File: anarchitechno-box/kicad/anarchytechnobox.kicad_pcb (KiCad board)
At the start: 4 copper layers, 97.2 x 116.3 mm, 102 parts, among them J2 Conn_01x03_Socket, J4 C2988369, Q1001 IRFS4310Z, Q1101 IRFS4310Z, Q1301 IRFS4310Z, Q1401 IRFS4310Z, Q201 12mhz, Q401 IRFS4310Z, Q501 IRFS4310Z, Q701 IRFS4310Z, Q801 IRFS4310Z, SW1 C318884, U1 TC4426xOA, U101 <value>, U2 ADuM1200AR, U201 TLV74311PDBVR, U21 C85364, U301 ADuM1200AR, U302 TC4426xOA, U4 LM7812_TO220, U401 ADuM1200AR, U402 TC4426xOA, U403 ADuM1200AR, U404 TC4426xOA, U6 TME-0503S, U67 LP5907MFX-3.3

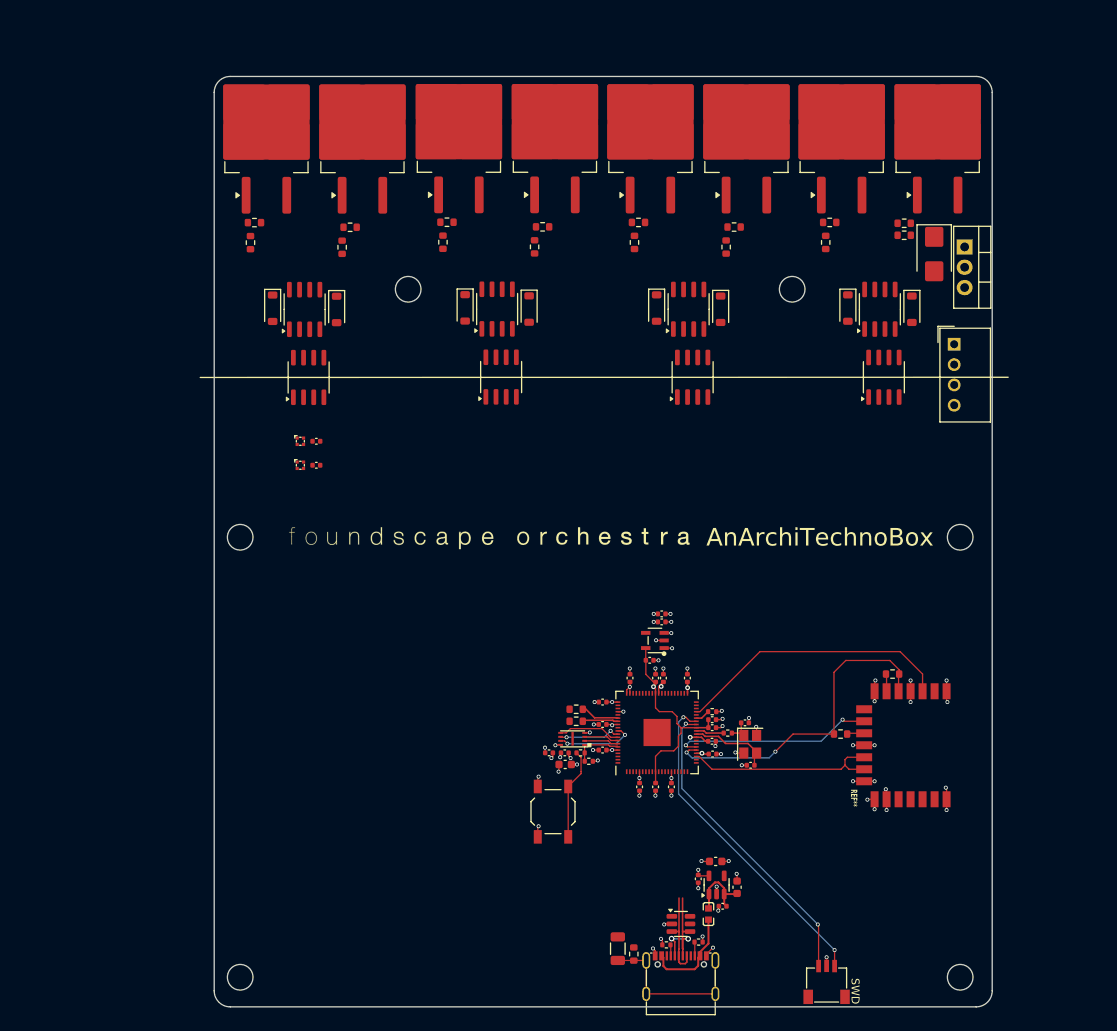
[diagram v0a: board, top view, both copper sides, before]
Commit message: Stijn in de Trein
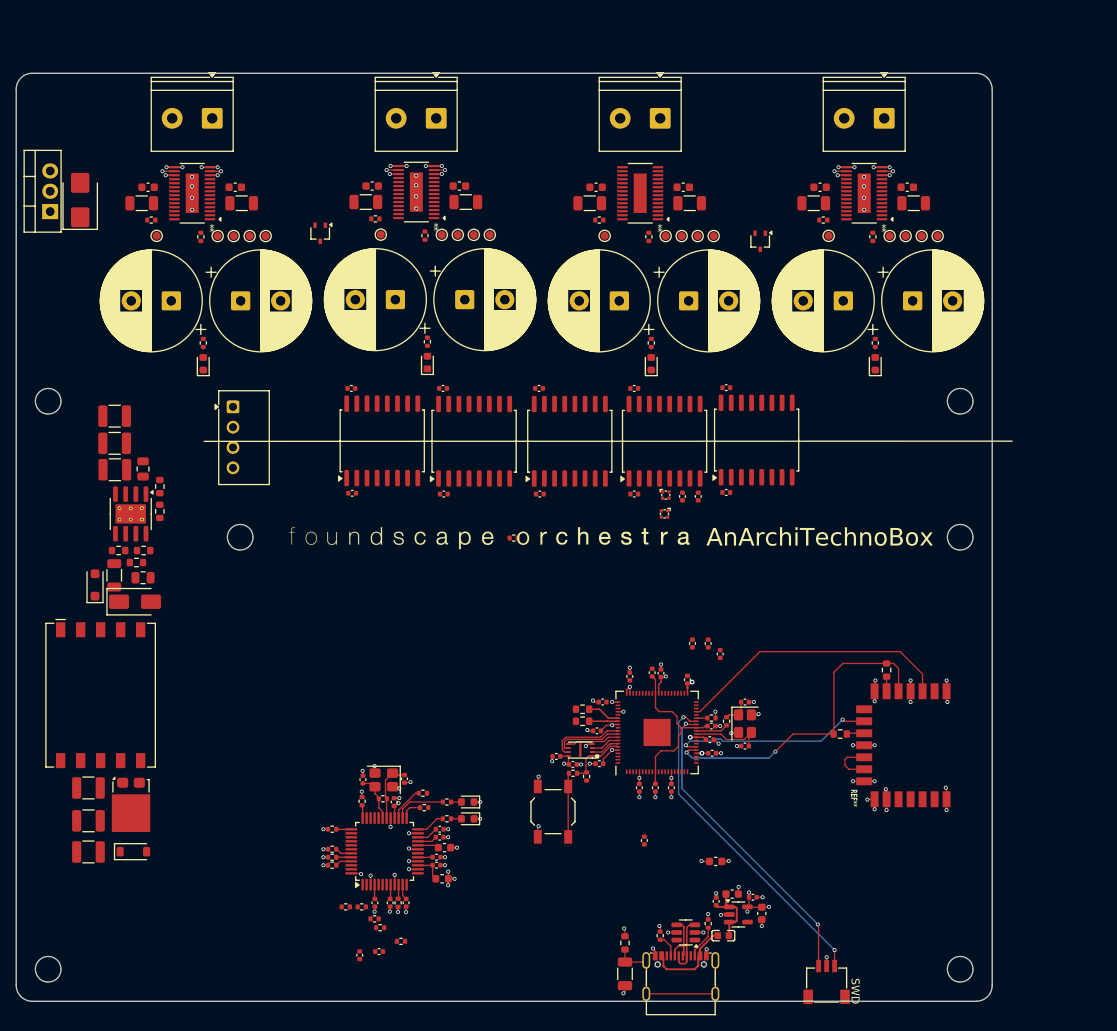
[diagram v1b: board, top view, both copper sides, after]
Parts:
- removed C101, C102: 100nF, Capacitor_SMD:C_0402_1005Metric
- removed C139, C140: 100n, Capacitor_SMD:C_0402_1005Metric
- removed C150: 4.7n 100v, Capacitor_SMD:C_1206_3216Metric
- removed D1004, D1104, D1304, D1404, D404, D504, D704, D804: MBR0530, Diode_SMD:D_SOD-123
- removed D101: C5349953, TinyLEDs:XL-1010
- removed H11, H12, H7, H8, H9: MountingHole, MountingHole:MountingHole_3.2mm_M3
- removed L3: BLM18PG121SN1D_C14709, BigFishImports:L0603
- removed Q1001, Q1101, Q1301, Q1401, Q401, Q501, Q701, Q801: IRFS4310Z, Package_TO_SOT_SMD:TO-263-2
- removed Q201: 12mhz, Crystal:Crystal_SMD_SeikoEpson_TSX3225-4Pin_3.2x2.5mm
- removed R1003, R1103, R1303, R1403, R403, R503, R703, R803: 100R, Resistor_SMD:R_0603_1608Metric
- removed R1004, R1104, R1304, R1404, R205, R404, R504, R704, R804: 10k, Resistor_SMD:R_0603_1608Metric
- removed R202: 27, Resistor_SMD:R_0603_1608Metric
- removed R204: 470, Resistor_SMD:R_0603_1608Metric
- removed U$2: C2843335 W25Q16JVUXIQ, ZephKicad:USON-8-EP(2x3)
- removed U2, U301, U401, U403: ADuM1200AR, Package_SO:SOIC-8_3.9x4.9mm_P1.27mm
- removed U201: TLV74311PDBVR, jlcpcb3:SOT-23-5_L3.0-W1.7-P0.95-LS2.8-BL
- removed U302, U402, U404: TC4426xOA, Package_SO:SOIC-8_3.9x4.9mm_P1.27mm
- removed the U4 at (137.6, 53.7)
- removed U6: TME-0503S, Converter_DCDC:Converter_DCDC_TRACO_TME_03xxS_05xxS_12xxS_Single_THT
- removed U67: LP5907MFX-3.3, Package_TO_SOT_SMD:SOT-23-5
- added C1: 100nF, Capacitor_SMD:C_0402_1005Metric, F.Cu at (102.3, 84.9)
- added C10: 1u, Capacitor_SMD:C_0402_1005Metric, F.Cu at (105.5, 103.3)
- added C11: 100nF, Capacitor_SMD:C_0402_1005Metric, F.Cu at (106.0, 117.0)
- added C12: 10uF, Capacitor_SMD:C_0603_1608Metric, F.Cu at (108.5, 134.6)
- added C13: 100nF, Capacitor_SMD:C_0402_1005Metric, F.Cu at (99.6, 107.0)
- added C15: 100nF, Capacitor_SMD:C_0402_1005Metric, F.Cu at (91.9, 118.3)
- added C17: 100n, Capacitor_SMD:C_0402_1005Metric, F.Cu at (111.1, 135.0)
- added C18: 1u, Capacitor_SMD:C_0402_1005Metric, F.Cu at (107.0, 104.6)
- added C19: 1u, Capacitor_SMD:C_0402_1005Metric, F.Cu at (97.5, 127.9)
- added C20: 10uF, Capacitor_SMD:C_0603_1608Metric, F.Cu at (112.2, 137.0)
- added C21: 100nF, Capacitor_SMD:C_0402_1005Metric, F.Cu at (105.9, 113.6)
- added C22: 100nF, Capacitor_SMD:C_0402_1005Metric, F.Cu at (98.9, 121.3)
- added C23: 100nF, Capacitor_SMD:C_0402_1005Metric, F.Cu at (98.5, 106.9)
- added C24: 4.7n 100v, Capacitor_SMD:C_1206_3216Metric, F.Cu at (95.1, 144.6)
- added C25: 0.1uF, Capacitor_SMD:C_0402_1005Metric, F.Cu at (86.5, 117.4)
- added C27: 100nF, Capacitor_SMD:C_0402_1005Metric, F.Cu at (88.6, 118.4)
- added C29: 27p, Capacitor_SMD:C_0402_1005Metric, F.Cu at (110.1, 116.1)
- added C30: 100nF, Capacitor_SMD:C_0402_1005Metric, F.Cu at (61.0, 84.5)
- added C31: 100nF, Capacitor_SMD:C_0402_1005Metric, F.Cu at (60.9, 71.4)
- added C32: 100nF, Capacitor_SMD:C_0402_1005Metric, F.Cu at (107.8, 84.4)
- added C34: 1uF 50V, Capacitor_SMD:C_0603_1608Metric, F.Cu at (130.4, 46.2)
- added C35: 1uF 50V, Capacitor_SMD:C_0603_1608Metric, F.Cu at (119.5, 46.2)
- added C36: 10uF 50V, Capacitor_SMD:C_1206_3216Metric, F.Cu at (131.2, 48.2)
- added C37: 10uF 50V, Capacitor_SMD:C_1206_3216Metric, F.Cu at (118.7, 48.2)
- added C38: 1000uF 50V, Capacitor_THT:CP_Radial_D12.5mm_P5.00mm, F.Cu at (122.4, 60.4)
- added C39: 1000uF 50V, Capacitor_THT:CP_Radial_D12.5mm_P5.00mm, F.Cu at (131.1, 60.4)
- added C40: 1uF 50V, Capacitor_SMD:C_0603_1608Metric, F.Cu at (102.4, 46.2)
- added C41: 1uF 50V, Capacitor_SMD:C_0603_1608Metric, F.Cu at (91.5, 46.2)
- added C42: 10uF 50V, Capacitor_SMD:C_1206_3216Metric, F.Cu at (103.2, 48.2)
- added C43: 10uF 50V, Capacitor_SMD:C_1206_3216Metric, F.Cu at (90.7, 48.2)
- added C44: 1000uF 50V, Capacitor_THT:CP_Radial_D12.5mm_P5.00mm, F.Cu at (94.4, 60.4)
- added C45: 1000uF 50V, Capacitor_THT:CP_Radial_D12.5mm_P5.00mm, F.Cu at (103.1, 60.4)
- added C46: 100nF, Capacitor_SMD:C_0402_1005Metric, F.Cu at (72.5, 84.6)
- added C47: 100nF, Capacitor_SMD:C_0402_1005Metric, F.Cu at (84.5, 84.6)
- added C48: 100nF, Capacitor_SMD:C_0402_1005Metric, F.Cu at (96.3, 84.6)
- added C49: 100nF, Capacitor_SMD:C_0402_1005Metric, F.Cu at (96.3, 71.4)
- added C50: 100nF, Capacitor_SMD:C_0402_1005Metric, F.Cu at (84.4, 71.4)
- added C6: 4.7u, Capacitor_SMD:C_0402_1005Metric, F.Cu at (103.5, 103.3)
- added C64: 10n, Capacitor_SMD:C_0402_1005Metric, F.Cu at (61.9, 142.2)
- added C67: 10uF 50V, Capacitor_SMD:C_1210_3225Metric, F.Cu at (31.3, 78.3)
- added C68: 1uF 25V, Capacitor_SMD:C_0805_2012Metric, F.Cu at (34.9, 81.5)
- added C69: 220pF, Capacitor_SMD:C_0805_2012Metric, F.Cu at (34.9, 95.1)
- added C7: 100nF, Capacitor_SMD:C_0402_1005Metric, F.Cu at (96.9, 121.3)
- added C70: 47uF 10V, Capacitor_SMD:C_1210_3225Metric, F.Cu at (28.0, 121.3)
- added C71: 47uF 10V, Capacitor_SMD:C_1210_3225Metric, F.Cu at (28.0, 125.5)
- added C72: 47uF 10V, Capacitor_SMD:C_1210_3225Metric, F.Cu at (28.0, 129.3)
- added C74: 1uF 50V, Capacitor_SMD:C_0603_1608Metric, F.Cu at (74.4, 46.1)
- added C75: 1uF 50V, Capacitor_SMD:C_0603_1608Metric, F.Cu at (63.5, 46.1)
- added C76: 10uF 50V, Capacitor_SMD:C_1206_3216Metric, F.Cu at (75.2, 48.1)
- added C77: 10uF 50V, Capacitor_SMD:C_1206_3216Metric, F.Cu at (62.7, 48.1)
- added C78: 1000uF 50V, Capacitor_THT:CP_Radial_D12.5mm_P5.00mm, F.Cu at (66.4, 60.3)
- added C79: 1000uF 50V, Capacitor_THT:CP_Radial_D12.5mm_P5.00mm, F.Cu at (75.1, 60.3)
- added C8: 100nF, Capacitor_SMD:C_0402_1005Metric, F.Cu at (100.9, 121.3)
- added C80: 1uF 50V, Capacitor_SMD:C_0603_1608Metric, F.Cu at (46.4, 46.2)
- added C81: 1uF 50V, Capacitor_SMD:C_0603_1608Metric, F.Cu at (35.5, 46.2)
- added C82: 10uF 50V, Capacitor_SMD:C_1206_3216Metric, F.Cu at (47.2, 48.2)
- added C83: 10uF 50V, Capacitor_SMD:C_1206_3216Metric, F.Cu at (34.7, 48.2)
- added C84: 1000uF 50V, Capacitor_THT:CP_Radial_D12.5mm_P5.00mm, F.Cu at (38.4, 60.4)
- added C85: 1000uF 50V, Capacitor_THT:CP_Radial_D12.5mm_P5.00mm, F.Cu at (47.1, 60.4)
- added C9: 100n, Capacitor_SMD:C_0402_1005Metric, F.Cu at (106.5, 135.5)
- added D10: SMAJ18A, Diode_SMD:D_SMA, F.Cu at (33.9, 98.1)
- added D11: CMMSH1-100, Diode_SMD:D_SOD-123F, F.Cu at (28.9, 96.0)
- added D12: V8PM10SHM3/I, Package_TO_SOT_SMD:TO-277A, F.Cu at (33.4, 123.5)
- added D13: CMHZ5232B, Diode_SMD:D_SOD-123, F.Cu at (33.6, 129.3)
- added D14: RED, LED_SMD:LED_0603_1608Metric, F.Cu at (70.4, 68.2)
- added D15: RED, LED_SMD:LED_0603_1608Metric, F.Cu at (42.4, 68.3)
- added D2: C5349953, TinyLEDs:XL-1010, F.Cu at (100.2, 84.7)
- added D4: BAT54AW, Package_TO_SOT_SMD:SOT-323_SC-70, F.Cu at (57.0, 52.0)
- added D5: BAT54AW, Package_TO_SOT_SMD:SOT-323_SC-70, F.Cu at (112.0, 53.0)
- added D6: RED, LED_SMD:LED_0603_1608Metric, F.Cu at (126.4, 68.3)
- added D7: RED, LED_SMD:LED_0603_1608Metric, F.Cu at (98.4, 68.3)
- added D8: RED, LED_SMD:LED_0603_1608Metric, F.Cu at (75.4, 125.2)
- added D9: RED, LED_SMD:LED_0603_1608Metric, F.Cu at (75.4, 123.1)
- added FB1: BLM18PG121SN1D, Inductor_SMD:L_0603_1608Metric, F.Cu at (72.2, 132.7)
- added H1: MountingHole, MountingHole:MountingHole_3.2mm_M3, F.Cu at (23.0, 73.0)
- added H2: MountingHole, MountingHole:MountingHole_3.2mm_M3, F.Cu at (137.0, 90.0)
- added H3: MountingHole, MountingHole:MountingHole_3.2mm_M3, F.Cu at (137.0, 73.0)
- added H4: MountingHole, MountingHole:MountingHole_3.2mm_M3, F.Cu at (137.0, 144.0)
- added H6: MountingHole, MountingHole:MountingHole_3.2mm_M3, F.Cu at (23.0, 144.0)
- added J3: Screw_Terminal_01x02, TerminalBlock_Phoenix:TerminalBlock_Phoenix_PT-1,5-2-5.0-H_1x02_P5.00mm_Horizontal, F.Cu at (71.5, 37.6)
- added J4: Screw_Terminal_01x02, TerminalBlock_Phoenix:TerminalBlock_Phoenix_PT-1,5-2-5.0-H_1x02_P5.00mm_Horizontal, F.Cu at (43.5, 37.6)
- added J5: Screw_Terminal_01x02, TerminalBlock_Phoenix:TerminalBlock_Phoenix_PT-1,5-2-5.0-H_1x02_P5.00mm_Horizontal, F.Cu at (127.5, 37.6)
- added J6: Screw_Terminal_01x02, TerminalBlock_Phoenix:TerminalBlock_Phoenix_PT-1,5-2-5.0-H_1x02_P5.00mm_Horizontal, F.Cu at (99.5, 37.6)
- added L1: BLM18PG121SN1D_C14709, BigFishImports:L0603, F.Cu at (107.4, 139.8)
- added Q1: 12mhz, Crystal:Crystal_SMD_SeikoEpson_TSX3225-4Pin_3.2x2.5mm, F.Cu at (110.1, 113.3)
- added R1: 470, Resistor_SMD:R_0603_1608Metric, F.Cu at (127.8, 106.6)
- added R10: 10k, Resistor_SMD:R_0402_1005Metric, F.Cu at (105.9, 112.6)
- added R11: 1k, Resistor_SMD:R_0402_1005Metric, F.Cu at (107.8, 113.0)
- added R12: 470R, Resistor_SMD:R_0402_1005Metric, F.Cu at (126.4, 65.7)
- added R13: 0R, Resistor_SMD:R_0402_1005Metric, F.Cu at (126.1, 52.4)
- added R14: TBD, Resistor_SMD:R_0402_1005Metric, F.Cu at (119.9, 50.3)
- added R15: 470R, Resistor_SMD:R_0402_1005Metric, F.Cu at (98.4, 65.7)
- added R16: 0R, Resistor_SMD:R_0402_1005Metric, F.Cu at (98.1, 52.4)
- added R19: 1MEG, Resistor_SMD:R_0402_1005Metric, F.Cu at (64.8, 122.7)
- added R2: 10k, Resistor_SMD:R_0603_1608Metric, F.Cu at (122.0, 114.6)
- added R20: 1K, Resistor_SMD:R_0402_1005Metric, F.Cu at (58.5, 131.0)
- added R21: 1K, Resistor_SMD:R_0402_1005Metric, F.Cu at (58.5, 130.0)
- added R22: 1K, Resistor_SMD:R_0402_1005Metric, F.Cu at (58.5, 129.0)
- added R23: 1K, Resistor_SMD:R_0402_1005Metric, F.Cu at (62.2, 123.0)
- added R24: 1K, Resistor_SMD:R_0402_1005Metric, F.Cu at (58.5, 126.5)
- added R27: 470R, Resistor_SMD:R_0402_1005Metric, F.Cu at (72.8, 123.1)
- added R29: 12.4k, Resistor_SMD:R_0402_1005Metric, F.Cu at (66.7, 135.7)
- added R3: 1M, Resistor_SMD:R_0603_1608Metric, F.Cu at (95.1, 140.7)
- added R30: 49R9, Resistor_SMD:R_0402_1005Metric, F.Cu at (62.2, 136.2)
- added R31: 49R9, Resistor_SMD:R_0402_1005Metric, F.Cu at (60.2, 136.2)
- added R32: 10R, Resistor_SMD:R_0402_1005Metric, F.Cu at (67.1, 140.5)
- added R36: 200K, Resistor_SMD:R_0603_1608Metric, F.Cu at (37.0, 83.7)
- added R37: 150K, Resistor_SMD:R_0603_1608Metric, F.Cu at (31.8, 91.7)
- added R38: 113K, Resistor_SMD:R_0603_1608Metric, F.Cu at (34.9, 91.7)
- added R39: 100R, Resistor_SMD:R_1206_3216Metric, F.Cu at (31.3, 94.8)
- added R4: 5.1k, Resistor_SMD:R_0402_1005Metric, F.Cu at (99.5, 139.8)
- added R40: 10K, Resistor_SMD:R_0603_1608Metric, F.Cu at (34.0, 93.2)
- added R41: 470R, Resistor_SMD:R_0402_1005Metric, F.Cu at (70.4, 65.6)
- added R42: 0R, Resistor_SMD:R_0402_1005Metric, F.Cu at (70.1, 52.3)
- added R43: TBD, Resistor_SMD:R_0402_1005Metric, F.Cu at (63.9, 50.2)
- added R44: 470R, Resistor_SMD:R_0402_1005Metric, F.Cu at (42.4, 65.7)
- added R45: 0R, Resistor_SMD:R_0402_1005Metric, F.Cu at (42.1, 52.4)
- added R46: TBD, Resistor_SMD:R_0402_1005Metric, F.Cu at (35.9, 50.3)
- added R5: 5.1k, Resistor_SMD:R_0402_1005Metric, F.Cu at (105.5, 138.3)
- added R6: 10k, Resistor_SMD:R_0402_1005Metric, F.Cu at (90.3, 119.9)
- added R7: 27, Resistor_SMD:R_0603_1608Metric, F.Cu at (89.8, 113.0)
- added R8: 27, Resistor_SMD:R_0603_1608Metric, F.Cu at (89.8, 111.5)
- added R9: 1k, Resistor_SMD:R_0402_1005Metric, F.Cu at (88.6, 119.5)
- added TP1: TestPoint, TestPoint:TestPoint_Pad_D1.0mm, F.Cu at (120.6, 52.3)
- added TP10: TestPoint, TestPoint:TestPoint_Pad_D1.0mm, F.Cu at (100.2, 52.3)
- added TP11: TestPoint, TestPoint:TestPoint_Pad_D1.0mm, F.Cu at (64.6, 52.2)
- added TP12: TestPoint, TestPoint:TestPoint_Pad_D1.0mm, F.Cu at (74.2, 52.2)
- added TP13: TestPoint, TestPoint:TestPoint_Pad_D1.0mm, F.Cu at (76.2, 52.2)
- added TP14: TestPoint, TestPoint:TestPoint_Pad_D1.0mm, F.Cu at (78.2, 52.2)
- added TP15: TestPoint, TestPoint:TestPoint_Pad_D1.0mm, F.Cu at (72.2, 52.2)
- added TP16: TestPoint, TestPoint:TestPoint_Pad_D1.0mm, F.Cu at (36.6, 52.3)
- added TP17: TestPoint, TestPoint:TestPoint_Pad_D1.0mm, F.Cu at (46.2, 52.3)
- added TP18: TestPoint, TestPoint:TestPoint_Pad_D1.0mm, F.Cu at (48.2, 52.3)
- added TP19: TestPoint, TestPoint:TestPoint_Pad_D1.0mm, F.Cu at (50.2, 52.3)
- added TP2: TestPoint, TestPoint:TestPoint_Pad_D1.0mm, F.Cu at (130.2, 52.3)
- added TP20: TestPoint, TestPoint:TestPoint_Pad_D1.0mm, F.Cu at (44.2, 52.3)
- added TP3: TestPoint, TestPoint:TestPoint_Pad_D1.0mm, F.Cu at (132.2, 52.3)
- added TP4: TestPoint, TestPoint:TestPoint_Pad_D1.0mm, F.Cu at (134.2, 52.3)
- added TP5: TestPoint, TestPoint:TestPoint_Pad_D1.0mm, F.Cu at (128.2, 52.3)
- added TP6: TestPoint, TestPoint:TestPoint_Pad_D1.0mm, F.Cu at (92.6, 52.3)
- added TP7: TestPoint, TestPoint:TestPoint_Pad_D1.0mm, F.Cu at (102.2, 52.3)
- added TP8: TestPoint, TestPoint:TestPoint_Pad_D1.0mm, F.Cu at (104.2, 52.3)
- added TP9: TestPoint, TestPoint:TestPoint_Pad_D1.0mm, F.Cu at (106.2, 52.3)
- added U$1: C2843335 W25Q16JVUXIQ, ZephKicad:USON-8-EP(2x3), F.Cu at (89.5, 116.6)
- added U10: ISO7740DWR, Package_SO:SOIC-16W_7.5x10.3mm_P1.27mm, F.Cu at (111.6, 77.8)
- added U11: DRV8243SQDGQRQ1, parts:TI_HVSSOP-28, F.Cu at (125.0, 47.0)
- added U12: DRV8243SQDGQRQ1, parts:TI_HVSSOP-28, F.Cu at (97.0, 47.0)
- added U13: ISO7740DWR, Package_SO:SOIC-16W_7.5x10.3mm_P1.27mm, F.Cu at (76.2, 78.0)
- added U14: ISO7740DWR, Package_SO:SOIC-16W_7.5x10.3mm_P1.27mm, F.Cu at (88.2, 78.0)
- added U15: ISO7742DWR, Package_SO:SOIC-16W_7.5x10.3mm_P1.27mm, F.Cu at (100.0, 78.0)
- added U16: W5500, Package_QFP:LQFP-48_7x7mm_P0.5mm, F.Cu at (65.0, 129.3)
- added U18: ADPL54203ES8E#PBF, Package_SO:SOIC-8-1EP_3.9x4.9mm_P1.27mm_EP2.41x3.81mm_ThermalVias, F.Cu at (33.3, 87.1)
- added U19: 750311564, parts:T_Wurth_WE-FB-EP13_16.36, F.Cu at (29.6, 109.7)
- added U20: DRV8243SQDGQRQ1, parts:TI_HVSSOP-28, F.Cu at (69.0, 46.9)
- added U3: LM7812_TO220, Package_TO_SOT_THT:TO-220-3_Vertical, F.Cu at (23.2, 49.3)
- added U5: LP5907MFX-3.3, Package_TO_SOT_SMD:SOT-23-5, F.Cu at (109.3, 137.2)
- added U7: C85364, Package_TO_SOT_SMD:SOT-23-6, F.Cu at (102.7, 139.4)
- added U9: ISO7740DWR, Package_SO:SOIC-16W_7.5x10.3mm_P1.27mm, F.Cu at (64.8, 78.0)
- added Y1: 25MHz, Crystal:Crystal_SMD_3225-4Pin_3.2x2.5mm, F.Cu at (65.0, 120.3)
- C14: value 0.1uF -> 100nF
- C16: value 10uF -> 100nF; footprint Capacitor_SMD:C_0603_1608Metric -> Capacitor_SMD:C_0402_1005Metric
- C28: value 10uF -> 27p; footprint Capacitor_SMD:C_0603_1608Metric -> Capacitor_SMD:C_0402_1005Metric
- C3, C5, C60: value 1u -> 100nF
- C52, C53: value 100nF -> 15p
- C57: value 100nF -> 10nF
- C59: value 4.7u -> 4.7uF; footprint Capacitor_SMD:C_0402_1005Metric -> Capacitor_SMD:C_0603_1608Metric
- C63: value 100nF -> 22n
- C65: value 27p -> 330uF 50V; footprint Capacitor_SMD:C_0402_1005Metric -> Capacitor_SMD:C_1210_3225Metric
- C66: value 27p -> 10uF 50V; footprint Capacitor_SMD:C_0402_1005Metric -> Capacitor_SMD:C_1210_3225Metric
- D1: value C5349953 -> SM6T24A; footprint TinyLEDs:XL-1010 -> Diode_SMD:D_SMB
- D3: value SM6T24A -> C5349953; footprint Diode_SMD:D_SMB -> TinyLEDs:XL-1010
- R17: value 10k -> TBD
- R18: value 1k -> 10K
- R25: value 10k -> 470R
- R26: value 1k -> 470R
- R28: value 27 -> 470R; footprint Resistor_SMD:R_0603_1608Metric -> Resistor_SMD:R_0402_1005Metric
- R33: value 1M -> 49R9; footprint Resistor_SMD:R_0603_1608Metric -> Resistor_SMD:R_0402_1005Metric
- R34: value 5.1k -> 49R9
- R35: value 5.1k -> 1MEG; footprint Resistor_SMD:R_0402_1005Metric -> Resistor_SMD:R_0603_1608Metric
- U1: value TC4426xOA -> TME-0503S; footprint Package_SO:SOIC-8_3.9x4.9mm_P1.27mm -> Converter_DCDC:Converter_DCDC_TRACO_TME_03xxS_05xxS_12xxS_Single_THT
- U21: value C85364 -> DRV8243SQDGQRQ1; footprint Package_TO_SOT_SMD:SOT-23-6 -> parts:TI_HVSSOP-28
- moved U21 109.9 mm to (41.0, 47.0), turned to 180 degrees
- moved C66 87.6 mm to (31.3, 81.6)
- moved C65 87.6 mm to (31.3, 74.9), turned to 180 degrees
- moved R35 86.2 mm to (37.0, 86.8), turned to -90 degrees
- moved R17 63.1 mm to (91.9, 50.3)
- moved C61 47.5 mm to (63.8, 135.7), turned to -90 degrees
- moved D3 46.8 mm to (100.0, 87.1)
- moved C60 46.3 mm to (65.7, 135.7), turned to -90 degrees
- moved C51 43.1 mm to (72.4, 71.4), turned to 0 degrees
- moved D1 43.1 mm to (27.0, 47.8), turned to 90 degrees
- moved C59 39.9 mm to (72.5, 128.8), turned to 0 degrees
- moved C55 37.4 mm to (71.5, 130.0), turned to 0 degrees
- moved C33 37.4 mm to (107.8, 71.3), turned to 0 degrees
- moved R34 36.6 mm to (63.8, 137.7), turned to 0 degrees
- moved R18 36.2 mm to (81.2, 90.1)
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- renumbered J4 to J1, U101 to U4, U3 to U8
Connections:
- C14 pad 1: +3V3 -> GND
- C14 pad 2: GND -> +3V3
- C16 pad 1: +3V3 -> GND
- C16 pad 2: GND -> +3V3
- C28 pad 1: /RP2350BMCU/5V_filtered -> Net-(Q1-X1)
- C33 pad 1: GND -> +3.3VP
- C33 pad 2: +1V1 -> GND2
- C5 pad 2: +1V1 -> +3V3
- C51 pad 1: GND -> +3.3VP
- C51 pad 2: +3V3 -> GND2
- C52 pad 1: GND -> Net-(U16-XI/CLKIN)
- C52 pad 2: +3V3 -> GND
- C53 pad 1: GND -> Net-(U16-XO)
- C53 pad 2: +3V3 -> GND
- C54 pad 1: GND -> +3V3
- C54 pad 2: +3V3 -> GND
- C55 pad 1: GND -> +3.3VA
- C55 pad 2: +3V3 -> GND
- C56 pad 1: GND -> +3.3VA
- C56 pad 2: +3V3 -> GND
- C57 pad 1: GND -> Net-(U16-1V2O)
- C57 pad 2: +3V3 -> GND
- C58 pad 1: GND -> +3.3VA
- C58 pad 2: +3V3 -> GND
- C59 pad 1: +3V3 -> Net-(U16-TOCAP)
- C60 pad 1: +1V1 -> +3.3VA
- C61 pad 1: +1V1 -> +3.3VA
- C62 pad 1: +1V1 -> +3.3VA
- C63 pad 2: +3V3 -> Net-(U17-TCT)
- C65 pad 1: Net-(Q201-X1) -> +VDC
- C65 pad 2: GND -> GND2
- C66 pad 1: Net-(Q201-X2) -> +VDC
- C66 pad 2: GND -> GND2
- D1 pad 1: Net-(D1-DO) -> +24V
- D1 pad 2: +3V3 -> GND2
- D3 pad 1: +24V -> unconnected-(D3-DO-Pad1)
- D3 pad 2: GND2 -> +3V3
- J1 pad A5: Net-(J4-CC1) -> Net-(J1-CC1)
- J1 pad B5: Net-(J4-CC2) -> Net-(J1-CC2)
- J1 pad SHELL1: Net-(C150-Pad2) -> Net-(C24-Pad2)
- J1 pad SHELL2: Net-(C150-Pad2) -> Net-(C24-Pad2)
- J1 pad SHELL3: Net-(C150-Pad2) -> Net-(C24-Pad2)
- J1 pad SHELL4: Net-(C150-Pad2) -> Net-(C24-Pad2)
- R17 pad 1: +3V3 -> /TwoIsolatedFETs1/HBridge_B/DRV_ISENSE
- R17 pad 2: /RP2350BMCU/RUN -> GND2
- R18 pad 1: Net-(Q201-X1) -> +3.3VP
- R18 pad 2: Net-(U3-XOUT) -> /Isolators/PWR_DRV_nFAULT_COMMON
- R25 pad 1: /RP2350BMCU/MEM_CS -> Net-(U16-SPDLED)
- R25 pad 2: +3V3 -> Net-(D8-A)
- R26 pad 1: /RP2350BMCU/MEM_CS -> Net-(U16-LINKLED)
- R26 pad 2: /RP2350BMCU/BOOTSEL_BUT -> Net-(U17-LEDG_A)
- R28 pad 1: /RP2350BMCU/USB_N -> Net-(U16-ACTLED)
- R28 pad 2: /RP2350BMCU/USB_PRE_N -> Net-(U17-LEDY_A)
- R33 pad 1: GND -> +3.3V
- R33 pad 2: Net-(C150-Pad2) -> /Ethernet/ETH_RX_P
- R34 pad 1: Net-(J4-CC1) -> +3.3V
- R34 pad 2: GND -> /Ethernet/ETH_RX_M
- R35 pad 1: Net-(J4-CC2) -> Net-(R35-+)
- R35 pad 2: GND -> +VDC
- U1 pad 1: unconnected-(U1-NC-Pad1) -> GND2
- U1 pad 2: Net-(U1-IN_A) -> +5V
- U1 pad 3: unconnected-(U1-GND-Pad3) -> GND
- U1 pad 4: Net-(U1-IN_B) -> +3.3V
- U21 pad 1: unconnected-(U21-IO1-Pad1) -> /Isolators/PWR_SPI_CLK
- U21 pad 2: GND -> /Isolators/PWR_SPI_CS2
- U21 pad 3: /RP2350BMCU/USB_P -> /TwoIsolatedFETs0/HBridge_B/PWM_2
- U21 pad 4: /RP2350BMCU/USB_N -> /TwoIsolatedFETs0/HBridge_B/PWM_1
- U21 pad 5: +3V3 -> /Isolators/PWR_PWM_B_OFF
- U21 pad 6: unconnected-(U21-IO4-Pad6) -> +VDC
- U8 pad 1: unconnected-(U3-GPIO4-Pad1) -> /RP2350BMCU/PWM2_A
- U8 pad 11: unconnected-(U3-GPIO12-Pad11) -> /RP2350BMCU/PWM6_A
- U8 pad 13: unconnected-(U3-GPIO14-Pad13) -> /RP2350BMCU/PWM7_A
- U8 pad 19: unconnected-(U3-GPIO19-Pad19) -> /Ethernet/SPI_MOSI
- U8 pad 20: unconnected-(U3-GPIO20-Pad20) -> /Ethernet/SPI_MISO
- U8 pad 21: unconnected-(U3-GPIO21-Pad21) -> /Ethernet/SPI_CS
- U8 pad 22: unconnected-(U3-GPIO22-Pad22) -> /Ethernet/SPI_SCK
- U8 pad 28: unconnected-(U3-GPIO27-Pad28) -> /Isolators/MCU_SPI_CLK
- U8 pad 3: unconnected-(U3-GPIO6-Pad3) -> /RP2350BMCU/PWM3_A
- U8 pad 30: Net-(Q201-X2) -> Net-(Q1-X2)
- U8 pad 31: Net-(U3-XOUT) -> Net-(U8-XOUT)
- U8 pad 36: unconnected-(U3-GPIO28-Pad36) -> /Isolators/MCU_SPI_MOSI
- U8 pad 38: unconnected-(U3-GPIO30-Pad38) -> /Isolators/MCU_SPI_MISO
- U8 pad 39: unconnected-(U3-GPIO31-Pad39) -> /Isolators/MCU_DRV_nFAULT_COMMON
- U8 pad 40: unconnected-(U3-GPIO32-Pad40) -> /RP2350BMCU/I2C0_SCL
- U8 pad 42: unconnected-(U3-GPIO33-Pad42) -> /RP2350BMCU/I2C0_SDA
- U8 pad 43: unconnected-(U3-GPIO34-Pad43) -> /RP2350BMCU/UART0_TX
- U8 pad 44: unconnected-(U3-GPIO35-Pad44) -> /RP2350BMCU/UART0_RX
- U8 pad 45: unconnected-(U3-GPIO36-Pad45) -> /RP2350BMCU/UART1_TX
- U8 pad 46: unconnected-(U3-GPIO37-Pad46) -> /RP2350BMCU/UART1_RX
- U8 pad 47: unconnected-(U3-GPIO38-Pad47) -> /RP2350BMCU/I2C1_SCL
- U8 pad 48: unconnected-(U3-GPIO39-Pad48) -> /RP2350BMCU/I2C1_SDA
- U8 pad 49: unconnected-(U3-GPIO40_ADC0-Pad49) -> /Isolators/MCU_PWM_A_OFF
- U8 pad 52: unconnected-(U3-GPIO41_ADC1-Pad52) -> /Isolators/MCU_CS1
- U8 pad 53: unconnected-(U3-GPIO42_ADC2-Pad53) -> /Isolators/MCU_PWM_B_OFF
- U8 pad 54: unconnected-(U3-GPIO43_ADC3-Pad54) -> /Isolators/MCU_CS2
- U8 pad 55: unconnected-(U3-GPIO44_ADC4-Pad55) -> /Isolators/MCU_PWM_C_OFF
- U8 pad 56: unconnected-(U3-GPIO45_ADC5-Pad56) -> /Isolators/MCU_CS3
- U8 pad 57: unconnected-(U3-GPIO46_ADC6-Pad57) -> /Isolators/MCU_PWM_D_OFF
- U8 pad 58: unconnected-(U3-GPIO47_ADC7-Pad58) -> /Isolators/MCU_CS4
- U8 pad 6: unconnected-(U3-GPIO8-Pad6) -> /RP2350BMCU/PWM4_A
- U8 pad 77: unconnected-(U3-GPIO0-Pad77) -> /RP2350BMCU/PWM0_A
- U8 pad 78: unconnected-(U3-GPIO1-Pad78) -> /LED_STRING
- U8 pad 79: /LED_STRING -> /RP2350BMCU/PMW1_A
- U8 pad 8: unconnected-(U3-GPIO10-Pad8) -> /RP2350BMCU/PWM5_A
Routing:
- net GND2: track 0.00 -> 26.8 mm, vias 0 -> 36
- net Net-(C24-Pad2): track 0.00 -> 21.0 mm
- net Net-(C150-Pad2): track 20.6 -> 0.00 mm
- net /RP2350BMCU/WIFI_23: track 25.3 -> 5.83 mm
- net GND: track 47.0 -> 63.7 mm, vias 51 -> 70
- net +3.3VA: track 0.00 -> 13.4 mm
- net Net-(Q201-X2): track 10.2 -> 0.00 mm
- net +3V3: track 33.9 -> 43.3 mm, vias 27 -> 31
- net Net-(Q1-X2): track 0.00 -> 8.92 mm
- net /RP2350BMCU/USB_N: track 14.5 -> 6.79 mm, vias 2 -> 0
- net Net-(U16-XI/CLKIN): track 0.00 -> 7.01 mm
- net Net-(U16-DUPLED): track 0.00 -> 6.51 mm
- net Net-(U16-XO): track 0.00 -> 5.25 mm
- net +1V1: track 26.7 -> 21.5 mm, vias 1 -> 0
- net Net-(U16-ACTLED): track 0.00 -> 4.39 mm
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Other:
- board size 97.2 x 116.3 mm -> 122 x 116 mm

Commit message: meer Stijn in de Trein
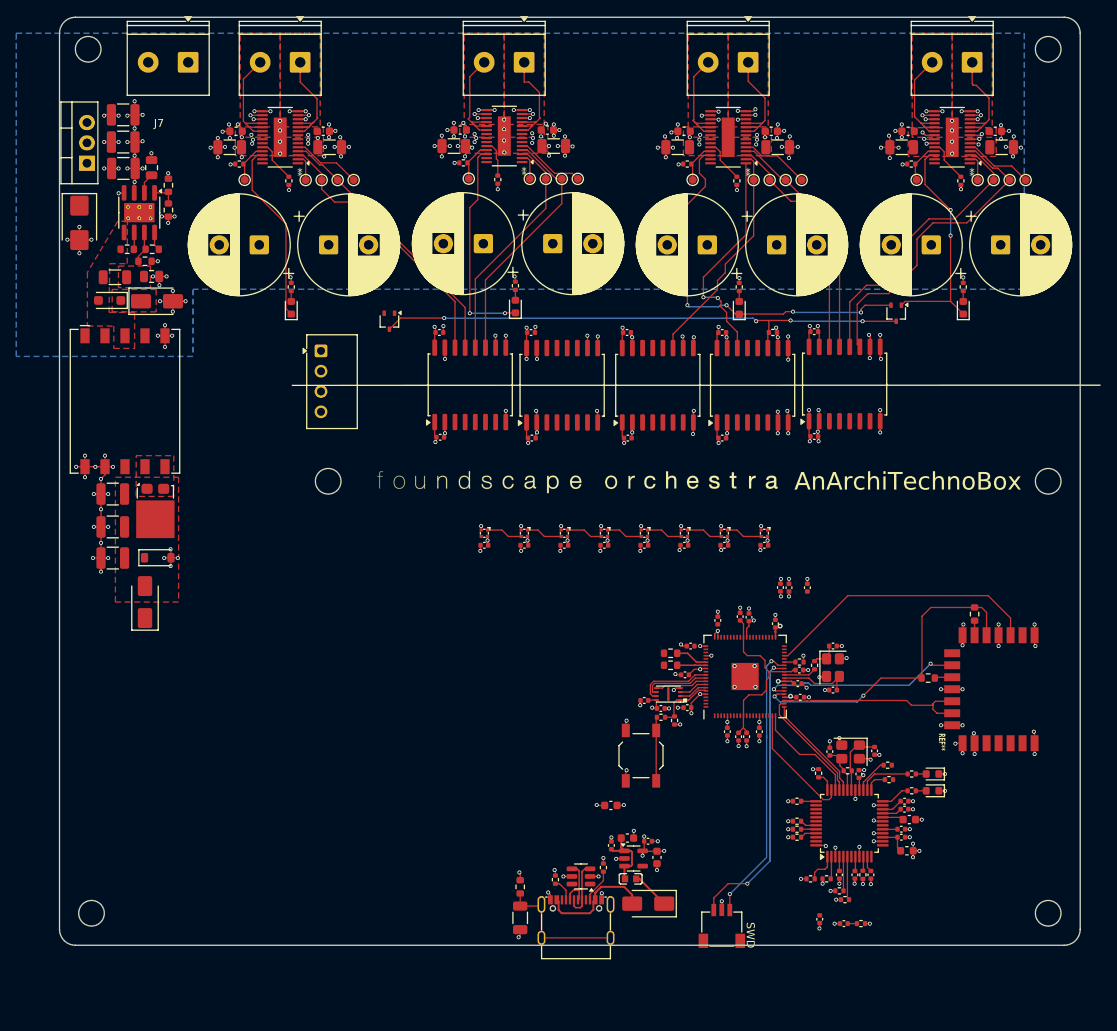
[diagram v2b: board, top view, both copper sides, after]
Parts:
- added C86: 100nF, Capacitor_SMD:C_0402_1005Metric, F.Cu at (87.5, 91.0)
- added C87: 100nF, Capacitor_SMD:C_0402_1005Metric, F.Cu at (92.5, 91.0)
- added C88: 100nF, Capacitor_SMD:C_0402_1005Metric, F.Cu at (97.5, 91.0)
- added C89: 100nF, Capacitor_SMD:C_0402_1005Metric, F.Cu at (102.5, 91.0)
- added C90: 100nF, Capacitor_SMD:C_0402_1005Metric, F.Cu at (107.5, 91.0)
- added C91: 100nF, Capacitor_SMD:C_0402_1005Metric, F.Cu at (112.5, 91.0)
- added D16: SS34, Diode_SMD:D_SMA, F.Cu at (98.0, 135.8)
- added D17: SS34, Diode_SMD:D_SMA, F.Cu at (35.1, 98.1)
- added D18: C5349953, TinyLEDs:XL-1010, F.Cu at (87.5, 89.5)
- added D19: C5349953, TinyLEDs:XL-1010, F.Cu at (92.5, 89.5)
- added D20: C5349953, TinyLEDs:XL-1010, F.Cu at (97.5, 89.5)
- added D21: C5349953, TinyLEDs:XL-1010, F.Cu at (102.5, 89.5)
- added D22: C5349953, TinyLEDs:XL-1010, F.Cu at (107.5, 89.5)
- added D23: C5349953, TinyLEDs:XL-1010, F.Cu at (112.5, 89.5)
- added J7: Screw_Terminal_01x02, TerminalBlock_Phoenix:TerminalBlock_Phoenix_PT-1,5-2-5.0-H_1x02_P5.00mm_Horizontal, F.Cu at (40.5, 30.6)
- moved C52 58.9 mm to (126.3, 116.7)
- moved C53 58.5 mm to (120.7, 116.8)
- moved Y1 58.5 mm to (123.3, 116.8)
- moved C54 58.2 mm to (124.3, 119.6)
- moved C58 58.2 mm to (125.8, 132.2)
- moved C60 58.2 mm to (123.8, 132.2)
- moved C63 58.2 mm to (122.5, 138.3)
- moved FB1 58.2 mm to (130.3, 129.2)
- moved R29 58.2 mm to (124.8, 132.2)
- moved R34 58.2 mm to (121.9, 134.2)
- moved U16 58.2 mm to (123.2, 125.8)
- moved C56 58.2 mm to (130.0, 124.0)
- moved C57 58.2 mm to (130.0, 123.0)
- moved D8 58.2 mm to (133.5, 121.7)
- moved D9 58.2 mm to (133.5, 119.6)
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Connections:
- net /TwoIsolatedFETs0/OUTPUT_A renamed /HB_1_OUT_A
- net /TwoIsolatedFETs0/OUTPUT_B renamed /HB_1_OUT_B
- net /TwoIsolatedFETs0/OUTPUT_C renamed /HB_1_OUT_C
- net /TwoIsolatedFETs0/OUTPUT_D renamed /HB_1_OUT_D
- net /TwoIsolatedFETs1/OUTPUT_A renamed /HB_2_OUT_A
- net /TwoIsolatedFETs1/OUTPUT_B renamed /HB_2_OUT_B
- net /TwoIsolatedFETs1/OUTPUT_C renamed /HB_2_OUT_C
- net /TwoIsolatedFETs1/OUTPUT_D renamed /HB_2_OUT_D
- net Net-(C69--) renamed /DCDC Flyback/VDC_CAPRES
- net Net-(D10-K) renamed /DCDC Flyback/VDC_DIODES
- net Net-(D11-A) renamed /DCDC Flyback/VDC_SW
- net Net-(D12-A-Pad1) renamed /DCDC Flyback/PRE_PRE_5V
- C30 pad 1: +3.3V -> +3V3
- C32 pad 1: +3.3V -> +3V3
- C46 pad 1: +3.3V -> +3V3
- C47 pad 1: +3.3V -> +3V3
- C48 pad 1: +3.3V -> +3V3
- C70 pad 1: +5V -> /DCDC Flyback/PRE_5V
- C71 pad 1: +5V -> /DCDC Flyback/PRE_5V
- C72 pad 1: +5V -> /DCDC Flyback/PRE_5V
- D12 pad 3: +5V -> /DCDC Flyback/PRE_5V
- D13 pad 1: +5V -> /DCDC Flyback/PRE_5V
- D14 pad 1: /TwoIsolatedFETs0/HBridge_A/DRV_nFAULT -> /TwoIsolatedFETs0/HBridge_B/DRV_nFAULT
- D15 pad 1: /TwoIsolatedFETs0/HBridge_B/DRV_nFAULT -> /TwoIsolatedFETs0/HBridge_A/DRV_nFAULT
- D3 pad 1: unconnected-(D3-DO-Pad1) -> Net-(D18-DI)
- D4 pad 1: /TwoIsolatedFETs0/HBridge_A/DRV_nFAULT -> /TwoIsolatedFETs0/HBridge_B/DRV_nFAULT
- D4 pad 2: /TwoIsolatedFETs0/HBridge_B/DRV_nFAULT -> /TwoIsolatedFETs0/HBridge_A/DRV_nFAULT
- D5 pad 1: /TwoIsolatedFETs1/HBridge_A/DRV_nFAULT -> /TwoIsolatedFETs1/HBridge_B/DRV_nFAULT
- D5 pad 2: /TwoIsolatedFETs1/HBridge_B/DRV_nFAULT -> /TwoIsolatedFETs1/HBridge_A/DRV_nFAULT
- D6 pad 1: /TwoIsolatedFETs1/HBridge_A/DRV_nFAULT -> /TwoIsolatedFETs1/HBridge_B/DRV_nFAULT
- D7 pad 1: /TwoIsolatedFETs1/HBridge_B/DRV_nFAULT -> /TwoIsolatedFETs1/HBridge_A/DRV_nFAULT
- J1 pad A4B9: +5V -> /RP2350BMCU/BREAKOUT_5V
- J1 pad A9B4: +5V -> /RP2350BMCU/BREAKOUT_5V
- R14 pad 1: /TwoIsolatedFETs1/HBridge_A/DRV_ISENSE -> /TwoIsolatedFETs1/HBridge_B/DRV_ISENSE
- R17 pad 1: /TwoIsolatedFETs1/HBridge_B/DRV_ISENSE -> /TwoIsolatedFETs1/HBridge_A/DRV_ISENSE
- R30 pad 1: +3.3V -> +3V3
- R31 pad 1: +3.3V -> +3V3
- R32 pad 1: +3.3V -> +3V3
- R33 pad 1: +3.3V -> +3V3
- R34 pad 1: +3.3V -> +3V3
- R43 pad 1: /TwoIsolatedFETs0/HBridge_A/DRV_ISENSE -> /TwoIsolatedFETs0/HBridge_B/DRV_ISENSE
- R46 pad 1: /TwoIsolatedFETs0/HBridge_B/DRV_ISENSE -> /TwoIsolatedFETs0/HBridge_A/DRV_ISENSE
- TP1 pad 1: /TwoIsolatedFETs1/HBridge_A/DRV_ISENSE -> /TwoIsolatedFETs1/HBridge_B/DRV_ISENSE
- TP11 pad 1: /TwoIsolatedFETs0/HBridge_A/DRV_ISENSE -> /TwoIsolatedFETs0/HBridge_B/DRV_ISENSE
- TP12 pad 1: /TwoIsolatedFETs0/HBridge_A/PWM_2 -> /TwoIsolatedFETs0/PWM_B_2
- TP13 pad 1: /TwoIsolatedFETs0/HBridge_A/PWM_1 -> /TwoIsolatedFETs0/PWM_B_1
- TP14 pad 1: /Isolators/PWR_PWM_A_OFF -> /Isolators/PWR_PWM_B_OFF
- TP16 pad 1: /TwoIsolatedFETs0/HBridge_B/DRV_ISENSE -> /TwoIsolatedFETs0/HBridge_A/DRV_ISENSE
- TP17 pad 1: /TwoIsolatedFETs0/HBridge_B/PWM_2 -> /TwoIsolatedFETs0/PWM_A_2
- TP18 pad 1: /TwoIsolatedFETs0/HBridge_B/PWM_1 -> /TwoIsolatedFETs0/PWM_A_1
- TP19 pad 1: /Isolators/PWR_PWM_B_OFF -> /Isolators/PWR_PWM_A_OFF
- TP2 pad 1: /TwoIsolatedFETs1/HBridge_A/PWM_2 -> /TwoIsolatedFETs1/PWM_B_2
- TP3 pad 1: /TwoIsolatedFETs1/HBridge_A/PWM_1 -> /TwoIsolatedFETs1/PWM_B_1
- TP4 pad 1: /Isolators/PWR_PWM_C_OFF -> /Isolators/PWR_PWM_D_OFF
- TP6 pad 1: /TwoIsolatedFETs1/HBridge_B/DRV_ISENSE -> /TwoIsolatedFETs1/HBridge_A/DRV_ISENSE
- TP7 pad 1: /TwoIsolatedFETs1/HBridge_B/PWM_2 -> /TwoIsolatedFETs1/PWM_A_2
- TP8 pad 1: /TwoIsolatedFETs1/HBridge_B/PWM_1 -> /TwoIsolatedFETs1/PWM_A_1
- TP9 pad 1: /Isolators/PWR_PWM_D_OFF -> /Isolators/PWR_PWM_C_OFF
- U10 pad 1: +3.3V -> +3V3
- U10 pad 11: /TwoIsolatedFETs1/HBridge_B/PWM_2 -> /TwoIsolatedFETs1/PWM_B_1
- U10 pad 12: /TwoIsolatedFETs1/HBridge_B/PWM_1 -> /TwoIsolatedFETs1/PWM_B_2
- U10 pad 13: /TwoIsolatedFETs1/HBridge_A/PWM_2 -> /TwoIsolatedFETs1/PWM_A_1
- U10 pad 14: /TwoIsolatedFETs1/HBridge_A/PWM_1 -> /TwoIsolatedFETs1/PWM_A_2
- U11 pad 25: /TwoIsolatedFETs1/HBridge_A/DRV_ISENSE -> /TwoIsolatedFETs1/HBridge_B/DRV_ISENSE
- U11 pad 26: /TwoIsolatedFETs1/HBridge_A/DRV_nFAULT -> /TwoIsolatedFETs1/HBridge_B/DRV_nFAULT
- U11 pad 3: /TwoIsolatedFETs1/HBridge_A/PWM_2 -> /TwoIsolatedFETs1/PWM_B_2
- U11 pad 4: /TwoIsolatedFETs1/HBridge_A/PWM_1 -> /TwoIsolatedFETs1/PWM_B_1
- U11 pad 5: /Isolators/PWR_PWM_C_OFF -> /Isolators/PWR_PWM_D_OFF
- U12 pad 25: /TwoIsolatedFETs1/HBridge_B/DRV_ISENSE -> /TwoIsolatedFETs1/HBridge_A/DRV_ISENSE
- U12 pad 26: /TwoIsolatedFETs1/HBridge_B/DRV_nFAULT -> /TwoIsolatedFETs1/HBridge_A/DRV_nFAULT
- U12 pad 3: /TwoIsolatedFETs1/HBridge_B/PWM_2 -> /TwoIsolatedFETs1/PWM_A_2
- U12 pad 4: /TwoIsolatedFETs1/HBridge_B/PWM_1 -> /TwoIsolatedFETs1/PWM_A_1
- U12 pad 5: /Isolators/PWR_PWM_D_OFF -> /Isolators/PWR_PWM_C_OFF
- U13 pad 1: +3.3V -> +3V3
- U14 pad 1: +3.3V -> +3V3
- U15 pad 1: +3.3V -> +3V3
- U15 pad 7: +3.3V -> +3V3
- U20 pad 25: /TwoIsolatedFETs0/HBridge_A/DRV_ISENSE -> /TwoIsolatedFETs0/HBridge_B/DRV_ISENSE
- U20 pad 26: /TwoIsolatedFETs0/HBridge_A/DRV_nFAULT -> /TwoIsolatedFETs0/HBridge_B/DRV_nFAULT
- U20 pad 3: /TwoIsolatedFETs0/HBridge_A/PWM_2 -> /TwoIsolatedFETs0/PWM_B_2
- U20 pad 4: /TwoIsolatedFETs0/HBridge_A/PWM_1 -> /TwoIsolatedFETs0/PWM_B_1
- U20 pad 5: /Isolators/PWR_PWM_A_OFF -> /Isolators/PWR_PWM_B_OFF
- U21 pad 25: /TwoIsolatedFETs0/HBridge_B/DRV_ISENSE -> /TwoIsolatedFETs0/HBridge_A/DRV_ISENSE
- U21 pad 26: /TwoIsolatedFETs0/HBridge_B/DRV_nFAULT -> /TwoIsolatedFETs0/HBridge_A/DRV_nFAULT
- U21 pad 3: /TwoIsolatedFETs0/HBridge_B/PWM_2 -> /TwoIsolatedFETs0/PWM_A_2
- U21 pad 4: /TwoIsolatedFETs0/HBridge_B/PWM_1 -> /TwoIsolatedFETs0/PWM_A_1
- U21 pad 5: /Isolators/PWR_PWM_B_OFF -> /Isolators/PWR_PWM_A_OFF
- U9 pad 1: +3.3V -> +3V3
- U9 pad 11: /TwoIsolatedFETs0/HBridge_B/PWM_2 -> /TwoIsolatedFETs0/PWM_B_1
- U9 pad 12: /TwoIsolatedFETs0/HBridge_B/PWM_1 -> /TwoIsolatedFETs0/PWM_B_2
- U9 pad 13: /TwoIsolatedFETs0/HBridge_A/PWM_2 -> /TwoIsolatedFETs0/PWM_A_1
- U9 pad 14: /TwoIsolatedFETs0/HBridge_A/PWM_1 -> /TwoIsolatedFETs0/PWM_A_2
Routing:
- net GND2: track 26.8 -> 130.4 mm, vias 36 -> 131
- net GND: track 63.7 -> 134.0 mm, vias 70 -> 134
- net /Isolators/PWR_DRV_nFAULT_COMMON: track 0.00 -> 67.7 mm, vias 0 -> 4
- net +VDC: track 0.00 -> 54.5 mm, vias 0 -> 66
- net /TwoIsolatedFETs1/HBridge_A/DRV_nFAULT: track 0.00 -> 47.9 mm, vias 0 -> 4
- net /TwoIsolatedFETs1/PWM_B_1: track 0.00 -> 39.3 mm
- net /TwoIsolatedFETs1/PWM_B_2: track 0.00 -> 36.4 mm
- net /TwoIsolatedFETs0/PWM_A_2: track 0.00 -> 34.1 mm
- net /TwoIsolatedFETs0/PWM_A_1: track 0.00 -> 34.0 mm
- net +3V3: track 43.3 -> 75.5 mm, vias 31 -> 56
- net /TwoIsolatedFETs0/PWM_B_1: track 0.00 -> 31.5 mm
- net +3.3VP: track 0.00 -> 30.1 mm, vias 0 -> 21
- net /TwoIsolatedFETs1/PWM_A_1: track 0.00 -> 30.1 mm
- net /TwoIsolatedFETs0/PWM_B_2: track 0.00 -> 29.5 mm
- net /TwoIsolatedFETs1/PWM_A_2: track 0.00 -> 29.3 mm
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- added copper zone on In2.Cu, net +3.3VP
- added copper zone on B.Cu, net +VDC
- added copper zone on F.Cu, net +VDC
- added copper zone on F.Cu, net /DCDC Flyback/PRE_5V
- added copper zone on F.Cu, net /DCDC Flyback/PRE_PRE_5V
- added copper zone on F.Cu, net /DCDC Flyback/VDC_CAPRES
- added copper zone on F.Cu, net /DCDC Flyback/VDC_DIODES
- added copper zone on F.Cu, net /DCDC Flyback/VDC_SW
- added copper zone on F.Cu, net /HB_1_OUT_A
- added copper zone on F.Cu, net /HB_1_OUT_B
- added copper zone on F.Cu, net /HB_1_OUT_C
- added copper zone on F.Cu, net /HB_1_OUT_D
- added copper zone on F.Cu, net /HB_2_OUT_A
- added copper zone on F.Cu, net /HB_2_OUT_B
- added copper zone on F.Cu, net /HB_2_OUT_C
- added copper zone on F.Cu, net /HB_2_OUT_D
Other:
- board size 122 x 116 mm -> 127.6 x 116 mm
